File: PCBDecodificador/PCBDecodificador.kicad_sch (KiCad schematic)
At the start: 2 parts, among them J1 Conector Mic 8 Vias, J2 Conector Mic 8 Vias

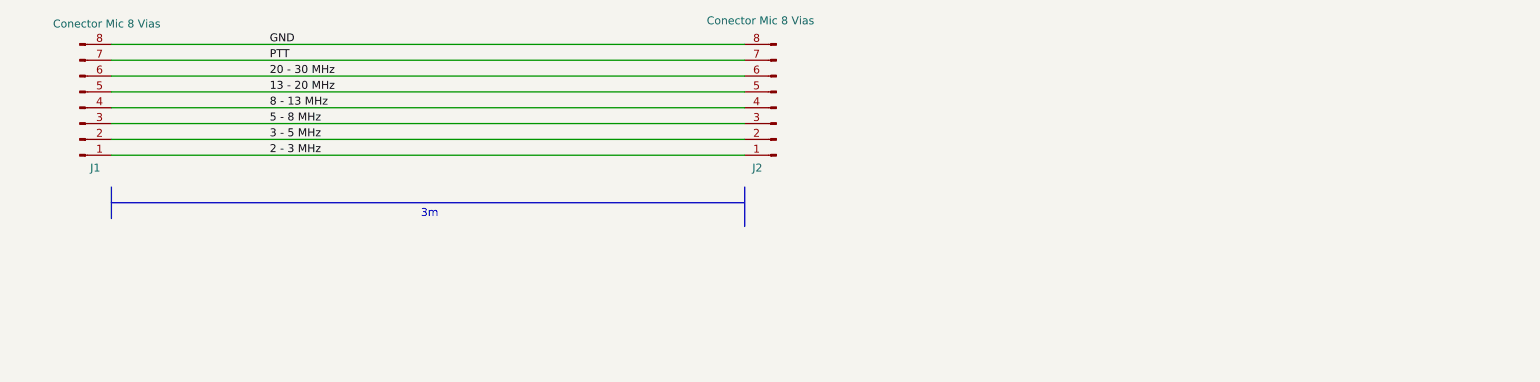
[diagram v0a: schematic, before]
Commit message: Adicionado PDF do Cabo Amplificador Decodificador
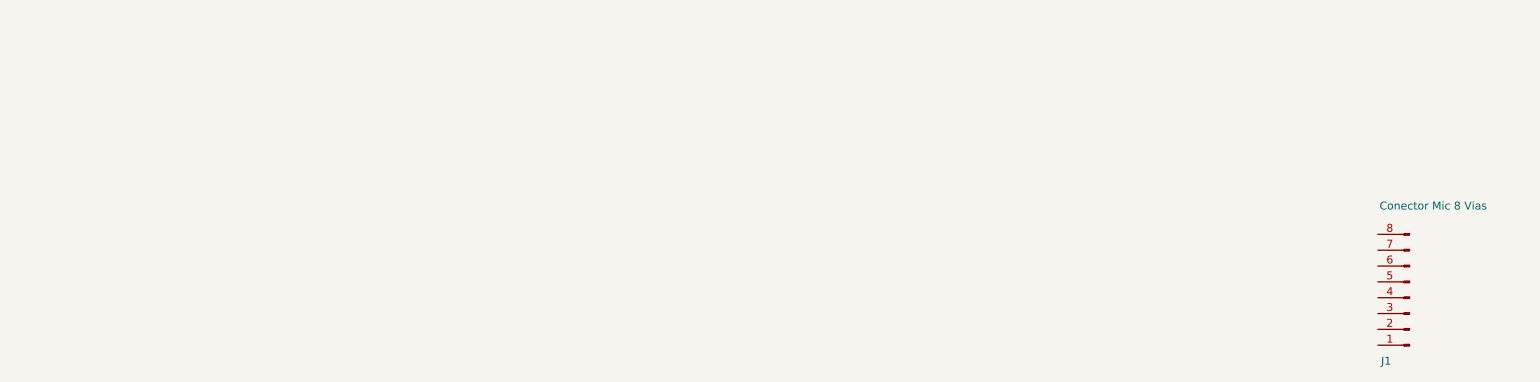
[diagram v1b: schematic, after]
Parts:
- removed J2: Conector Mic 8 Vias, symbol Connector:Conn_01x08_Pin
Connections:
- net 13 - 20 MHz: no longer names the net of J1.5 (Pin_5)
- net 2 - 3 MHz: no longer names the net of J1.1 (Pin_1)
- net 20 - 30 MHz: no longer names the net of J1.6 (Pin_6)
- net 3 - 5 MHz: no longer names the net of J1.2 (Pin_2)
- net 5 - 8 MHz: no longer names the net of J1.3 (Pin_3)
- net 8 - 13 MHz: no longer names the net of J1.4 (Pin_4)
- net GND: no longer names the net of J1.8 (Pin_8)
- net PTT: no longer names the net of J1.7 (Pin_7)
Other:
- note removed: "3m"
- title: Cabo Amplificador Decodificador -> PCB Decodificador
